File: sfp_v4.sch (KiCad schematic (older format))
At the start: 75 parts, among them J102 SMA, J104 SMA, J106 SMA, P101 SFP-CONNECTOR, P103 CONN_01X01, P106 CONN_01X01, T101 ADT2-1T, T102 ADT2-1T, U101 LMH6702, U102 LMH6702, U103 LMH6702, U104 74HC14

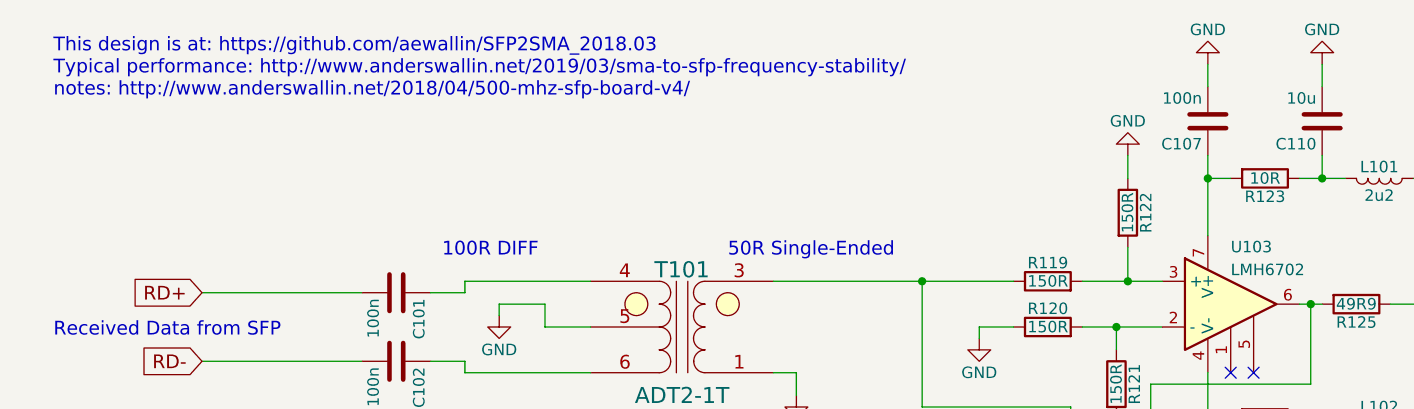
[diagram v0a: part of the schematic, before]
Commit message: minor tuning
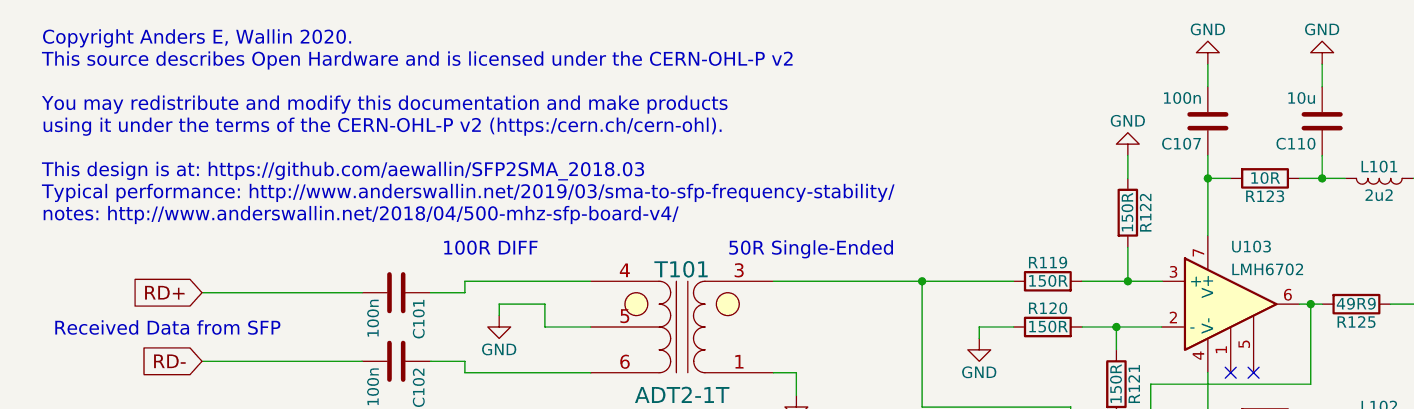
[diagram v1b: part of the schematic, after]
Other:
- note added: "Copyright Anders E, Wallin 2020.\nThis source describes Open Hardware and is licensed under the CERN-OHL-P v2\n\nYou may redistribute and modify this documentation and make products\nusing it under the terms of the CERN-OHL-P v2 (https:/cern.ch/cern-ohl).\n\nThis design is at: https://github.com/aewallin/SFP2SMA_2018.03\nTypical performance: http://www.anderswallin.net/2019/03/sma-to-sfp-frequenc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"
- note removed: "This design is at: https://github.com/aewallin/SFP2SMA_2018.03\nTypical performance: http://www.anderswallin.net/2019/03/sma-to-sfp-frequency-stability/\nnotes: http://www.anderswallin.net/2018/04/500-mhz-sfp-board-v4/\n"
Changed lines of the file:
@@
 NoConn ~ 6900 5200
 NoConn ~ 6800 5200
-Text Notes 700  900  0    60   ~ 0
-This design is at: https://github.com/aewallin/SFP2SMA_2018.03\nTypical performance: http://www.anderswallin.net/2019/03/sma-to-sfp-frequency-stability/\nnotes: http://www.anderswallin.net/2018/04/500-mhz-sfp-board-v4/\n
+Text Notes 650  1450 0    60   ~ 0
+Copyright Anders E, Wallin 2020.\nThis source describes Open Hardware and is licensed under the CERN-OHL-P v2\n\nYou may redistribute and modify this documentation and make products\nusing it under the terms of the CERN-OHL-P v2 (https:/cern.ch/cern-ohl).\n\nThis design is at: https://github.com/aewallin/SFP2SMA_2018.03\nTypical performance: http://www.anderswallin.net/2019/03/sma-to-sfp-frequency-stability/\nnotes: http://www.anderswallin.net/2018/04/500-mhz-sfp-board-v4/\n
 $Comp
 L 74xx:74HC14 U104
